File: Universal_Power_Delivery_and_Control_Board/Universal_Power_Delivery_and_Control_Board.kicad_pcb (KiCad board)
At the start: 4 copper layers, 123 parts, among them CN1 B03B-XASK-1-A(LF)(SN), CN2 B03B-XASK-1-A(LF)(SN), CN3 B03B-XASK-1-A(LF)(SN), CN4 B03B-XASK-1-A(LF)(SN), Q2 AO3401A, U1 TPS259470LRPWR, U10 SN74LVC1G17DCKR, U11 SN74LVC1G17DCKR, U12 SN74LVC1G17DCKR, U13 SN74LVC1G17DCKR, U14 SN74LVC1G17DCKR, U15 SN74LVC541APWR_C113281, U16 SN74LVC541APWR_C113281, U17 SN74LVC1G17DCKR, U19 TF-0803-0, U2 CH224Q_C46061833, U20 TCA9555PWR, U3 USBLC6-2SC6, U4 ESD2CAN24-ES, U5 S2B-ZR (LF)(SN), U6 USBLC6-2SC6, U7 TPS54202DDC, U8 TPS51385RJNR, U9 TPS24751RUVR

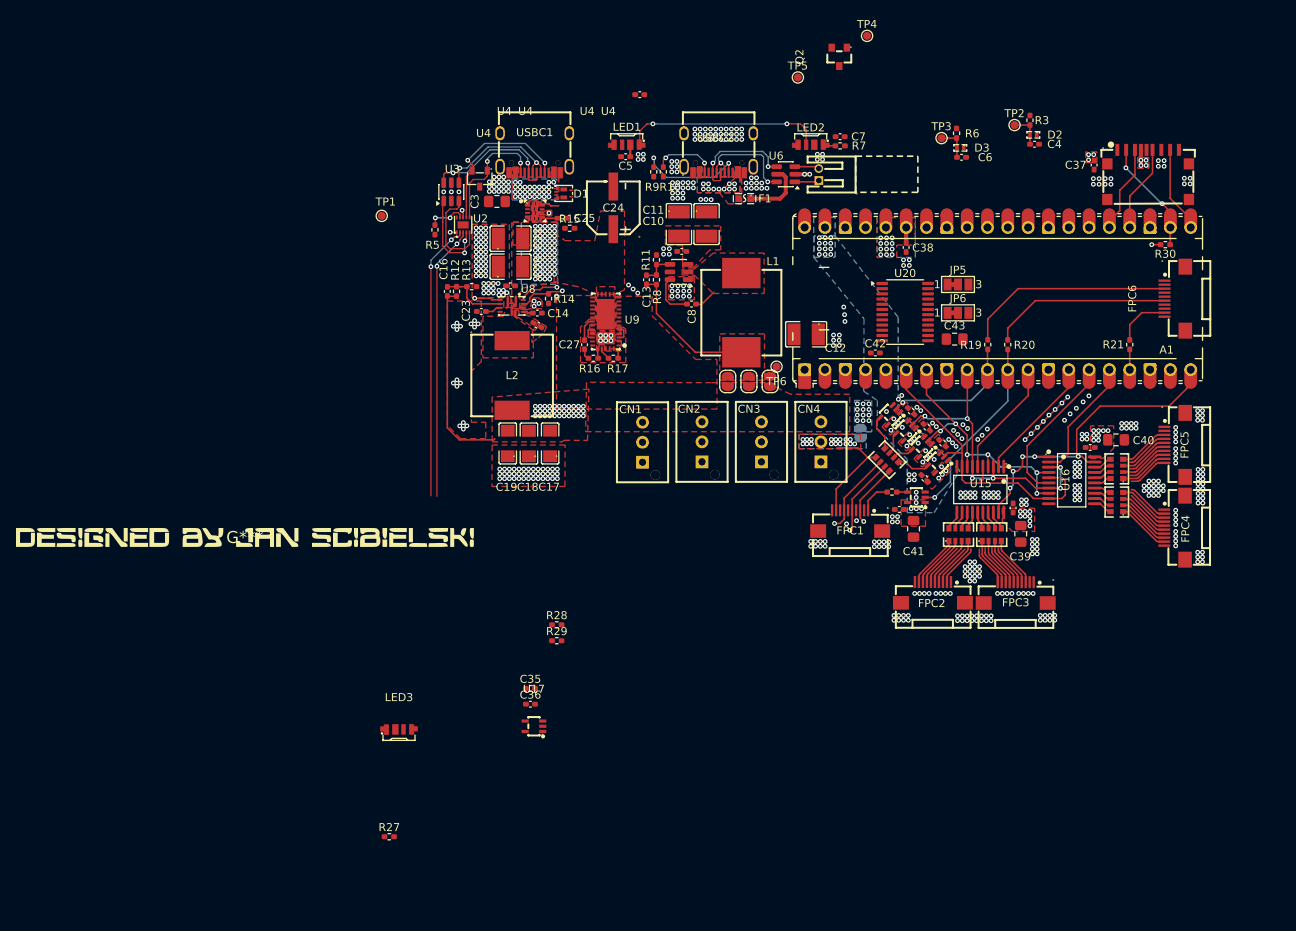
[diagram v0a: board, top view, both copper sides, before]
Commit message: Added some misc stuff layout almost finished.
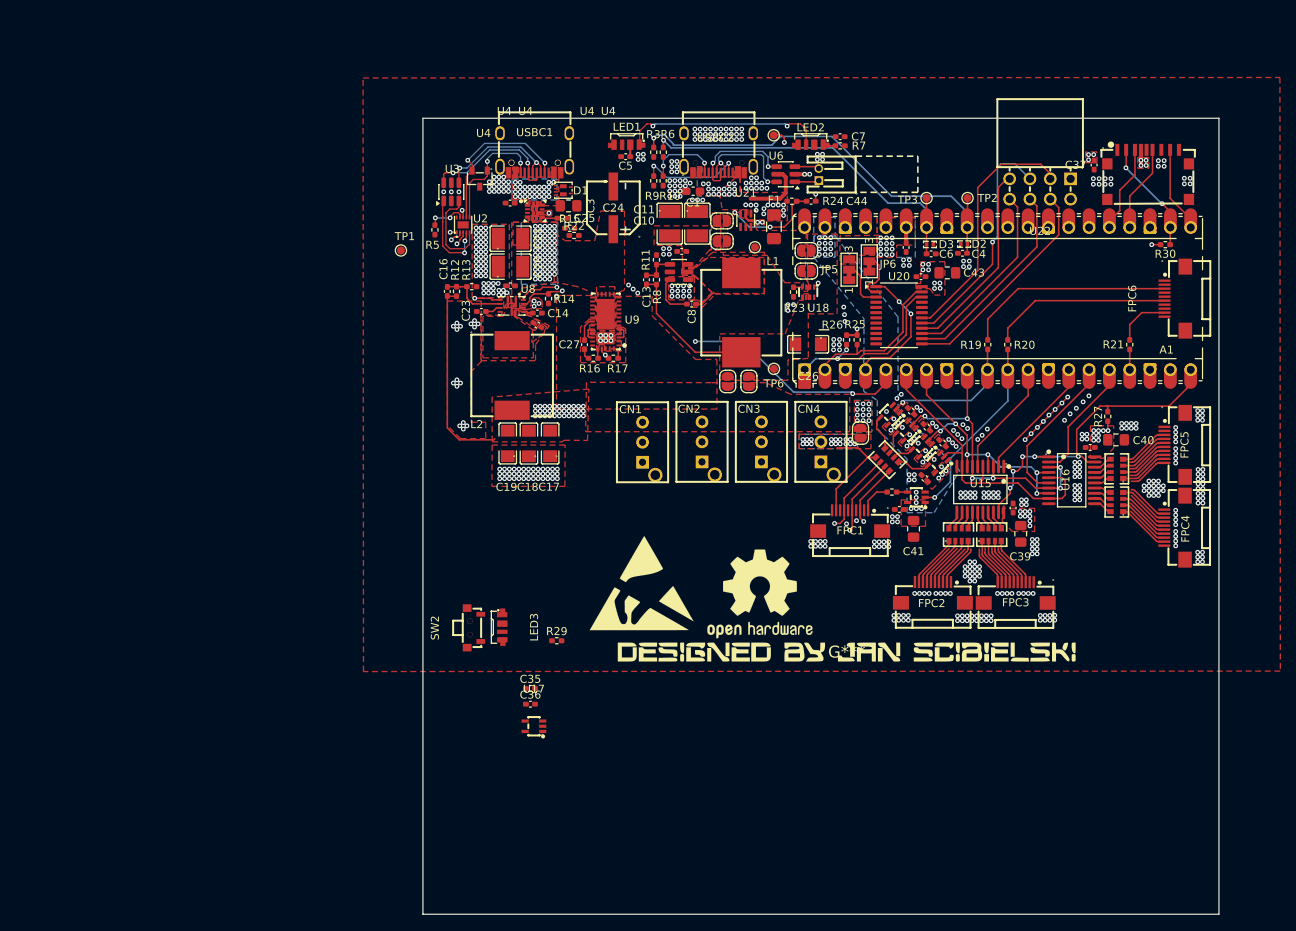
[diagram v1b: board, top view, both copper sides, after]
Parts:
- removed C12: 47uF, lcsc_footprints:C77101_C1210
- removed JP3: SolderJumper_2_Open, Jumper:SolderJumper-2_P1.3mm_Open_RoundedPad1.0x1.5mm
- removed Q2: AO3401A, lcsc_footprints:C15127_SOT-23_L2_9-W1_3-P1_90-LS2_4-BR
- removed R28: 33R, Resistor_SMD:R_0402_1005Metric_Pad0.72x0.64mm_HandSolder
- added C1: 1uF, Capacitor_SMD:C_0603_1608Metric_Pad1.08x0.95mm_HandSolder, F.Cu at (135.9, 47.3)
- added C26: 47uF, lcsc_footprints:C426659_C1206, F.Cu at (150.3, 66.5)
- added C44: 10nF, Capacitor_SMD:C_0402_1005Metric_Pad0.74x0.62mm_HandSolder, F.Cu at (150.7, 48.6)
- added JP10: SolderJumper_2_Open, Jumper:SolderJumper-2_P1.3mm_Open_RoundedPad1.0x1.5mm, F.Cu at (139.5, 53.6)
- added JP7: SolderJumper_2_Open, Jumper:SolderJumper-2_P1.3mm_Open_RoundedPad1.0x1.5mm, F.Cu at (150.1, 57.3)
- added JP8: SolderJumper_2_Open, Jumper:SolderJumper-2_P1.3mm_Open_RoundedPad1.0x1.5mm, F.Cu at (150.1, 54.8)
- added JP9: SolderJumper_2_Open, Jumper:SolderJumper-2_P1.3mm_Open_RoundedPad1.0x1.5mm, F.Cu at (139.5, 51.0)
- added R22: ?, Resistor_SMD:R_0402_1005Metric_Pad0.72x0.64mm_HandSolder, F.Cu at (121.0, 52.9)
- added R23: 1K, Resistor_SMD:R_0402_1005Metric_Pad0.72x0.64mm_HandSolder, F.Cu at (148.5, 59.9)
- added R24: 1K, Resistor_SMD:R_0402_1005Metric_Pad0.72x0.64mm_HandSolder, F.Cu at (148.3, 48.6)
- added R25: 4.7K, Resistor_SMD:R_0402_1005Metric_Pad0.72x0.64mm_HandSolder, F.Cu at (156.4, 65.9)
- added R26: 4.7K, Resistor_SMD:R_0402_1005Metric_Pad0.72x0.64mm_HandSolder, F.Cu at (155.1, 65.9)
- added REF**: OSHW-Logo2_14.6x12mm_SilkScreen, Symbol:OSHW-Logo2_14.6x12mm_SilkScreen, F.Cu at (144.3, 97.7)
- added REF**: ESD-Logo_13.2x12mm_SilkScreen, Symbol:ESD-Logo_13.2x12mm_SilkScreen, F.Cu at (129.5, 96.3)
- added SW2: TS1102-TD35HBM, lcsc_footprints:C36936640_SW-SMD_TS1102-TD35HBM, F.Cu at (108.5, 101.9)
- added U18: LM66200DRLR, lcsc_footprints:C3235556_SOT-583-8_L2_1-W1_2-P0_50-LS1_6-BL, F.Cu at (150.3, 59.9)
- added U21: TPS22919DCK, Package_TO_SOT_SMD:SOT-363_SC-70-6, F.Cu at (142.5, 51.0)
- added U22: HC-PM254-8.5H-2X4PW-02A, lcsc_footprints:C42163146_HDR-TH_8P-P2_54-H-F-R2-C4-S2_54-W8_5, F.Cu at (179.3, 47.0)
- F1: value 06H1100D -> Fuse; footprint lcsc_footprints:C182303_F0603 -> Fuse:Fuse_1206_3216Metric_Pad1.42x1.75mm_HandSolder
- JP4: moved to F.Cu
- R11, R15: value 13.3K -> ?
- R3, R6: value 1K -> 4.7K
- moved R27 104.0 mm to (187.8, 75.5), turned to 90 degrees
- moved G*** 76.6 mm to (155.1, 104.9)
- moved R3 47.2 mm to (131.0, 42.4), turned to 90 degrees
- moved R6 36.7 mm to (132.2, 42.4), turned to 90 degrees
- moved TP4 29.9 mm to (143.7, 54.3)
- moved C2 21.1 mm to (113.0, 48.8), turned to 180 degrees
- moved LED3 18.2 mm to (112.1, 101.8), turned to -90 degrees
- moved C4 16.3 mm to (169.6, 55.1), turned to 180 degrees
- moved D2 16.2 mm to (169.8, 53.9), turned to 0 degrees
- moved JP5 13.7 mm to (155.4, 57.1), turned to 90 degrees
- moved JP6 12.8 mm to (157.9, 56.1), turned to 90 degrees
- moved C6 12.7 mm to (165.7, 55.1)
- moved D3 12.7 mm to (165.5, 54.0)
- moved C42 11.1 mm to (164.4, 58.0), turned to 180 degrees
- moved TP2 10.9 mm to (170.2, 48.2)
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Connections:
- net /Power_Output/5V_O1 renamed /Digital_Signal_Output/CLK
- net /Power_Output/5V_O2 renamed /Digital_Signal_Output/LE
- net /Power_Output/5V_O3 renamed /Digital_Signal_Output/OE
- A1 pad 1: /SCL -> /SDA
- A1 pad 2: /SDA -> /SCL
- A1 pad 5: unconnected-(A1-GPIO3-Pad5) -> /SS_EN
- C10 pad 2: Net-(U7-VIN) -> +12V_PD
- C11 pad 2: Net-(U7-VIN) -> +12V_PD
- C9 pad 1: Net-(U7-VIN) -> +12V_PD
- CN1 pad : (no net) -> GND
- CN2 pad : (no net) -> GND
- CN3 pad : (no net) -> GND
- CN4 pad : (no net) -> GND
- F1 pad 1: +5V_VBUS -> /PD_Section/VBUS
- F1 pad 2: Net-(F1-Pad2) -> Net-(U21-IN)
- R15 pad 2: unconnected-(R15-Pad2) -> Net-(R15-Pad2)
- R17 pad 1: /Power_Output/SOFT_START_EN -> /SS_EN
- R29 pad 1: Net-(R28-Pad2) -> Net-(U17-Y)
- TP4 pad 1: +5V_VBUS -> /PD_Section/VBUS
- U20 pad 13: unconnected-(U20-P10-Pad13) -> Net-(U20-P10)
- U20 pad 14: unconnected-(U20-P11-Pad14) -> Net-(U20-P11)
- U20 pad 15: unconnected-(U20-P12-Pad15) -> Net-(U20-P12)
- U20 pad 16: unconnected-(U20-P13-Pad16) -> Net-(U20-P13)
- U20 pad 17: unconnected-(U20-P14-Pad17) -> Net-(U20-P14)
- U20 pad 18: unconnected-(U20-P15-Pad18) -> Net-(U20-P15)
- U20 pad 4: unconnected-(U20-P00-Pad4) -> /P00
- U20 pad 5: unconnected-(U20-P01-Pad5) -> /P01
- U20 pad 6: unconnected-(U20-P02-Pad6) -> /P02
- U20 pad 7: unconnected-(U20-P03-Pad7) -> /P03
- U20 pad 8: unconnected-(U20-P04-Pad8) -> /P04
- U20 pad 9: unconnected-(U20-P05-Pad9) -> /P05
- U6 pad 5: +5V_VBUS -> Net-(U21-IN)
- U7 pad 3: Net-(U7-VIN) -> +12V_PD
- U9 pad 33: /Power_Output/SOFT_START_EN -> /SS_EN
- USBC2 pad A4B9: Net-(F1-Pad2) -> Net-(U21-IN)
- USBC2 pad B4A9: Net-(F1-Pad2) -> Net-(U21-IN)
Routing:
- net /PD_Section/CC1_read: track 4.33 -> 53.6 mm, vias 0 -> 1
- net /PD_Section/CC2_read: track 4.33 -> 46.0 mm, vias 0 -> 1
- net /SS_EN: track 0.00 -> 41.5 mm, vias 0 -> 3
- net Net-(U20-P15): track 0.00 -> 31.2 mm
- net Net-(U20-P14): track 0.00 -> 29.3 mm, vias 0 -> 1
- net Net-(U20-P10): track 0.00 -> 27.6 mm
- net Net-(U20-P11): track 0.00 -> 25.5 mm
- net Net-(U20-P13): track 0.00 -> 24.6 mm
- net Net-(U20-P12): track 0.00 -> 23.6 mm
- net /INT: track 0.00 -> 16.5 mm, vias 0 -> 2
- net /SCL: track 34.8 -> 21.4 mm, vias 2 -> 1
- net Net-(U21-ON): track 0.00 -> 12.8 mm, vias 0 -> 2
- net GND: track 91.6 -> 102.2 mm, vias 457 -> 497
- net /SDA: track 34.3 -> 24.5 mm, vias 2 -> 3
- net Net-(U21-IN): track 0.00 -> 7.97 mm, vias 0 -> 28
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- added copper zone on F.Cu, net /PD_Section/VBUS
- added copper zone on B.Cu, net Net-(U21-IN)
- added copper zone on F.Cu, net Net-(U21-IN)
- removed copper zone on B.Cu, net Net-(F1-Pad2)
- removed copper zone on F.Cu, net Net-(F1-Pad2)
- removed copper zone on F.Cu, net Net-(U7-VIN)
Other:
- board outline added: 99.5 x 99.5 mm
